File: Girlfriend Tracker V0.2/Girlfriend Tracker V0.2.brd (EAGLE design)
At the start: 51.9 x 22 mm, 62 parts, among them IC1 SAM-M8Q, U1 3.6V/200mA - TLV70036DDCR, U2 3.6V/200mA - TLV70036DDCR, U3 ATSAMD21G-A, U4 3.6V/200mA - TLV70036DDCR, X1 SMA-142-0701-851/861, Y1 26MHz, Y2 32.768kHz

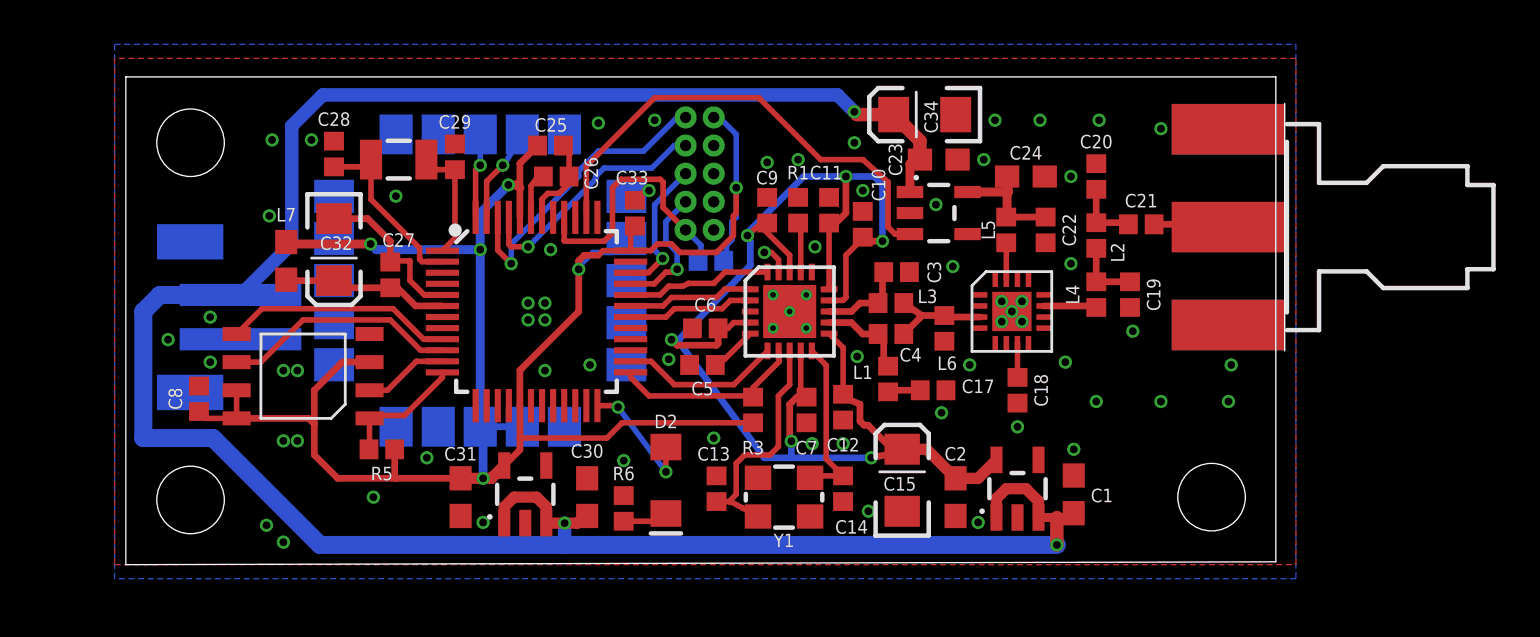
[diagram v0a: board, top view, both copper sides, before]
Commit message: girlfriend tracker board updates
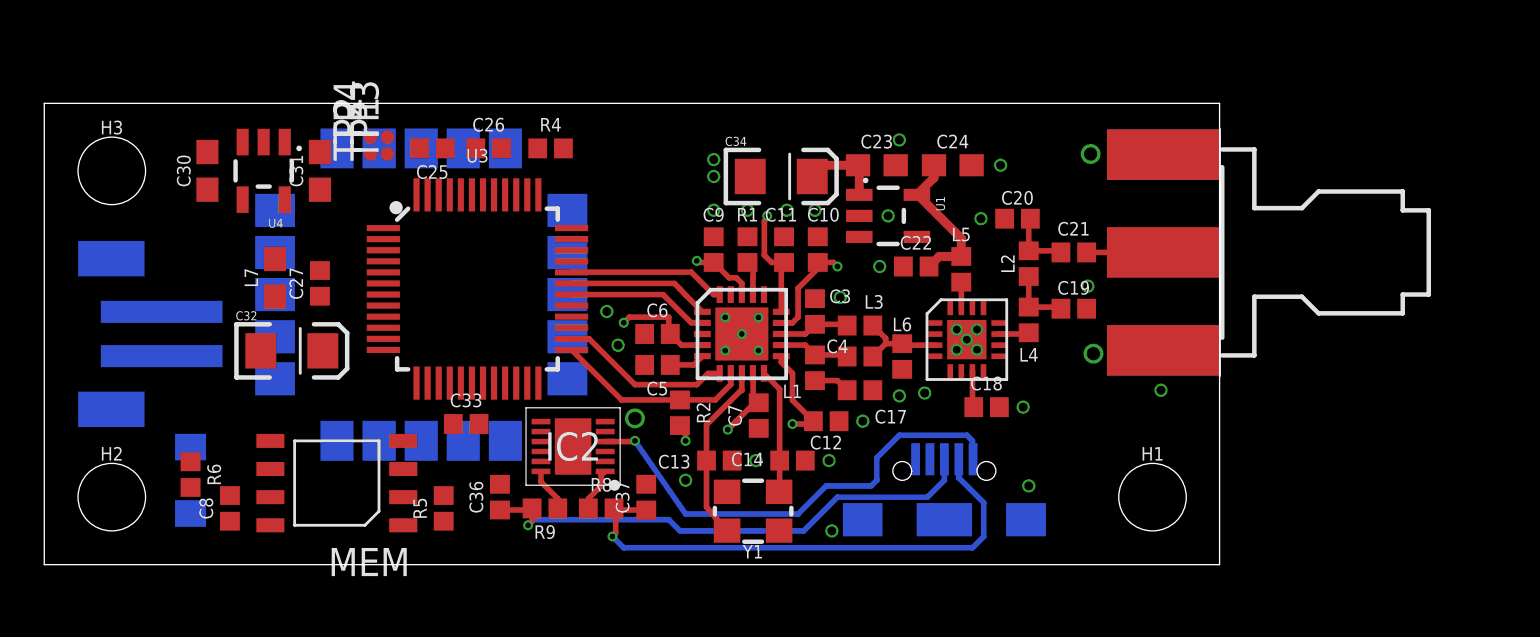
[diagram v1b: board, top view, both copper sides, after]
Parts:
- removed C1, C2: 2.2uF, SparkFun-Capacitors:0603
- removed C15: 10uF, SparkFun:EIA3216
- removed C28, C29: 15pF, SparkFun-Capacitors:0402
- removed JP1: CORTEX_DEBUG_PTH, SparkFun-Connectors:2X5-PTH-1.27MM
- removed R3: 10k, SparkFun-Resistors:0402
- removed U2: 3.6V/200mA - TLV70036DDCR, SparkFun-IC-Power:SOT23-5
- removed Y2: 32.768kHz, SparkFun-Clocks:CRYSTAL-SMD-3.2X1.5MM
- added C36, C37: 47pF, SparkFun-Capacitors:0402
- added IC2: FT234XD, ft234xd:SON45P300X300X80-13N
- added JP2: USB-MICROB", SparkFun-Connectors:USB-B-MICRO-SMD_V03
- added R2: (no value), SparkFun-Resistors:0402
- added R8, R9: 27, SparkFun-Resistors:0402
- added TP1, TP2, TP3, TP4: TPSQTP06R, testpad:TP06R
- C10, C7: value 10nF -> 0.1uF
- C11, C12, C17, C21, C9: value 220pF -> 0.1uF
- C13, C14: value 15pF -> 0.1uF
- C18, C22: value 0.01uF -> 0.1uF
- C19: value 8.2pF -> 0.1uF
- C20: value 5.6pF -> 0.1uF
- C24: value 0.1uF -> 2.2uF
- C26: value 1uF -> 0.1uF
- C3, C4: value 3.9pF -> 0.1uF
- C5, C6: value 100nF -> 0.1uF
- L2: value 27NH -> 6.8NH
- L4: value 22NH -> 6.8NH
- R1: value 56k -> (none)
- R5: value 10k -> (none)
- R6: value 63 -> (none)
- moved C30 22.6 mm to (7.37, 17.8)
- moved D2 21.5 mm to (6.60, 3.81), flipped to the bottom
- moved R6 19.6 mm to (6.60, 4.06)
- moved U4 18.8 mm to (9.91, 17.8), turned to 180 degrees
- moved H2 16.4 mm to (3.05, 3.05)
- moved C31 16.0 mm to (12.4, 17.8), turned to 90 degrees
- moved H3 15.3 mm to (3.05, 17.8)
- moved C33 12.2 mm to (19.1, 6.35), turned to 0 degrees
- moved R4 8.84 mm to (22.9, 18.8), flipped to the top, turned to 0 degrees
- moved C34 7.05 mm to (33.3, 17.5), turned to 0 degrees
- moved C22 6.07 mm to (39.4, 13.5), turned to 180 degrees
- moved C25 5.34 mm to (17.5, 18.8), turned to 180 degrees
- moved C8 5.15 mm to (8.38, 2.54)
- moved MEM 5.06 mm to (13.2, 4.32)
- moved C32 4.95 mm to (11.2, 9.65), turned to 0 degrees
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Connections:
- removed net N$14: C29.2, U3.1, Y2.P$2
- removed net N$15: C28.2, U3.2, Y2.P$1
- new net D+: IC2.12, R9.1
- new net D-: IC2.1, R8.1
- new net N$17: C37.1, JP2.D-1, R8.2
- new net N$2: C36.1, JP2.D+1, R9.2
- new net N$25: IC2.7
- new net N$26: IC2.10
- new net N$27: IC2.8
- new net N$28: IC2.11
- new net USB_VIN: IC2.4, JP2.VBUS1
- net !RESET: now also TP3.TP; no longer JP1.10
- net 3.3V: now also C10.2, C11.2, C12.2, C6.2, C7.2, C9.2, R2.2, U$1.11, U$1.14, U$1.15, U$1.18, U$1.4, U$1.9; no longer JP1.1, R3.1
- net CS_TX: now also R2.1; no longer R3.2
- net GND: now also C36.2, C37.2, IC2.13, IC2.5, JP2.GND1, JP2.SHIELD1, JP2.SHIELD2, JP2.SHIELD3, TP4.TP; no longer C1.2, C15.C, C2.2, C28.1, C29.1, JP1.3, JP1.5, U2.2
- net RX: no longer JP1.6
- net SWCLK: now also TP1.TP; no longer JP1.4
- net SWDIO: now also TP2.TP; no longer JP1.2
- net TX: no longer JP1.8
- net VDD: now also IC2.2, IC2.3, IC2.9; no longer C10.2, C11.2, C12.2, C15.A, C2.1, C6.2, C7.2, C9.2, U$1.11, U$1.14, U$1.15, U$1.18, U$1.4, U$1.9, U2.5
- net V_BATT: no longer C1.1, U2.1, U2.3
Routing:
- net V_BATT: track 108.8 -> 3.64 mm, vias 3 -> 0
- net 3.3V: track 95.6 -> 26.7 mm, vias 6 -> 7
- net VDD: track 66.0 -> 0.00 mm, vias 6 -> 0
- net N$17: track 0.00 -> 23.9 mm, vias 0 -> 1
- net N$2: track 0.00 -> 23.3 mm, vias 0 -> 1
- net AMP_EM: track 21.7 -> 0.00 mm
- net USB_VIN: track 0.00 -> 21.3 mm, vias 0 -> 1
- net GND: track 16.3 -> 0.00 mm, vias 59 -> 0
- net SWDIO: track 13.6 -> 0.00 mm, vias 1 -> 0
- net !RESET: track 12.2 -> 0.00 mm
- net SWCLK: track 11.2 -> 0.00 mm, vias 1 -> 0
- net SER0_SCK: track 10.6 -> 0.00 mm
- net SER0_MOSI: track 10.3 -> 0.00 mm
- net N$15: track 8.29 -> 0.00 mm, vias 0 -> 1
- net N$13: track 7.70 -> 0.00 mm
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- removed copper zone on layer 1, net GND
- removed copper zone on layer 16, net GND
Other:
- board size 51.9 x 22 mm -> 53.1 x 20.8 mm
- board text removed: "Girlfriend Tracker V0.1"
